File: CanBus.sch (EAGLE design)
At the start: 38 parts, among them IC1 MCP2515-I/SO, IC2 MEGA8-P, IC3 MCP2515-I/SO, Q1 16MHz, Q2 16MHz, Q3 16MHz, U1 MCP2562-E/SN, U2 MCP2562-E/SN, X1 MAC64L

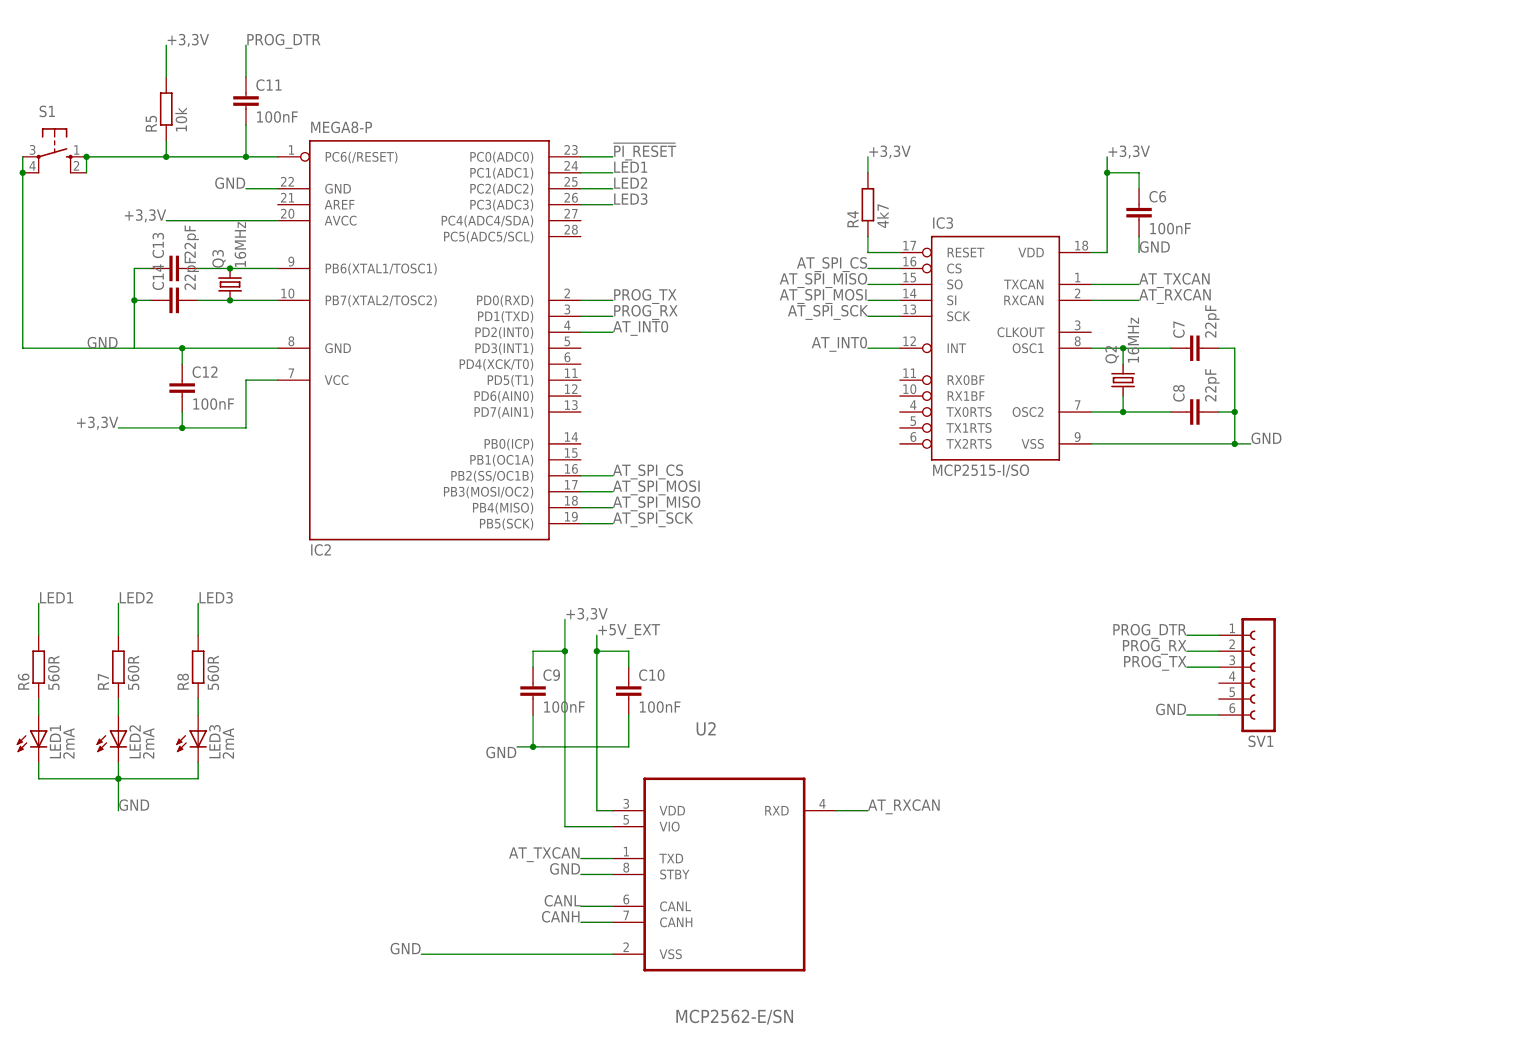
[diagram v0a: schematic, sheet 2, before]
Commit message: Platinen angepasst, Backplane
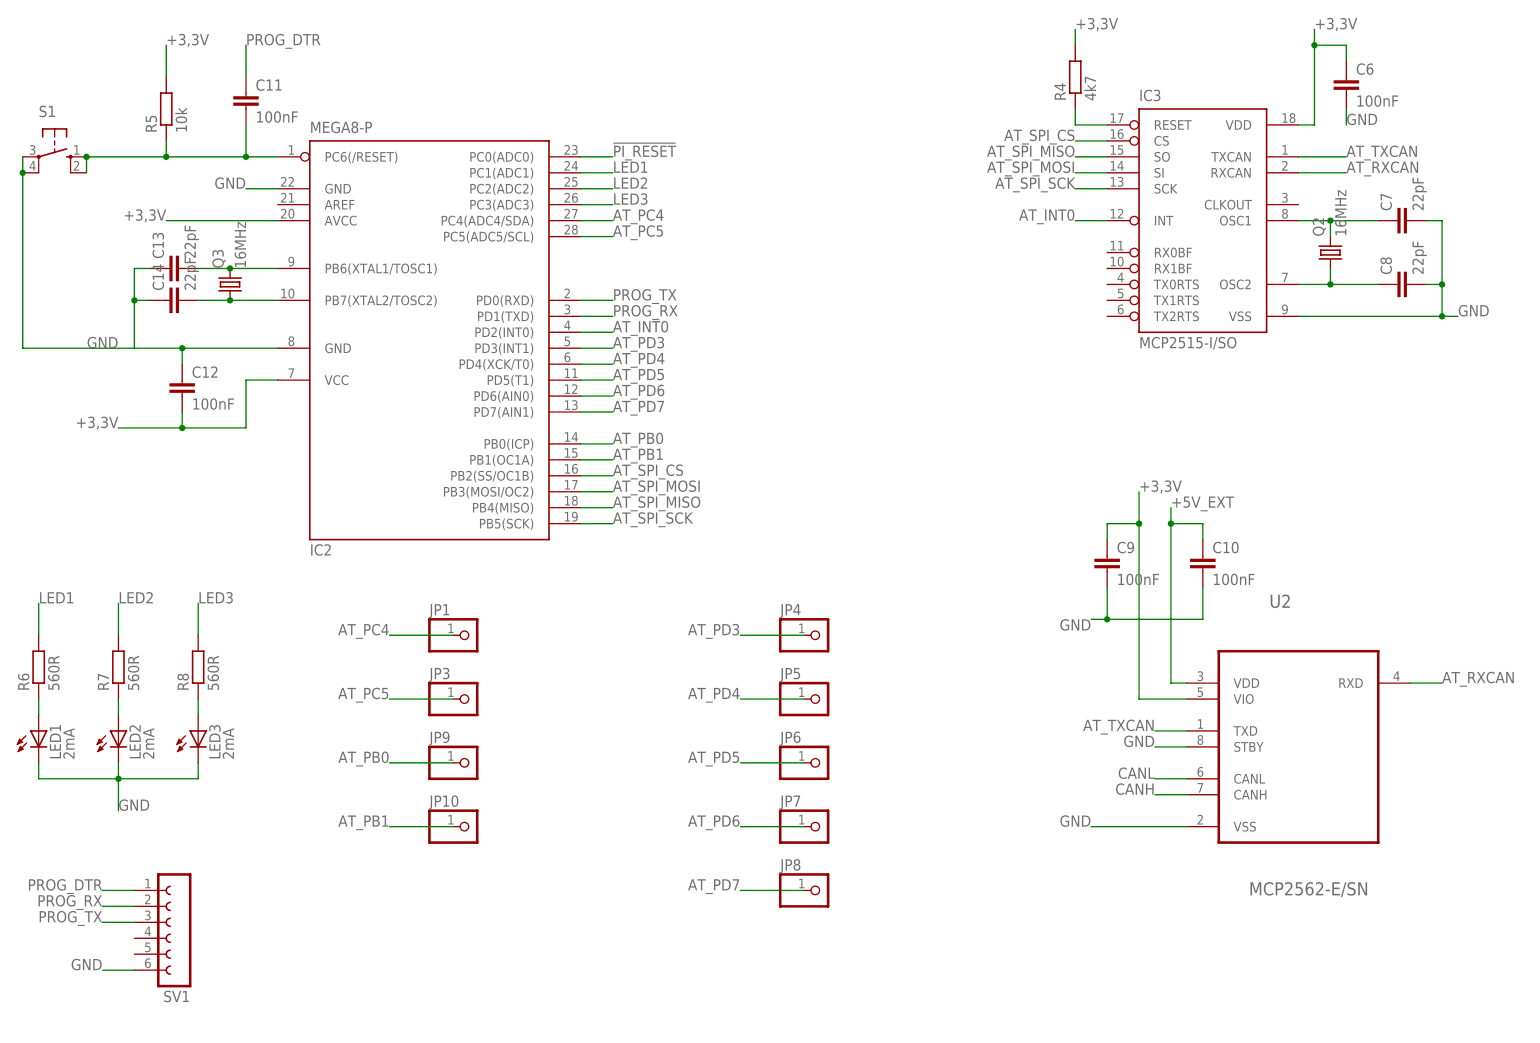
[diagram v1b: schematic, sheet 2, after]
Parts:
- added JP1, JP10, JP3, JP4, JP5, JP6, JP7, JP8, JP9: (no value), pinhead:PINHD-1X1
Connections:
- new net AT_PB0: IC2.PB0(ICP), JP9.1
- new net AT_PB1: IC2.PB1(OC1A), JP10.1
- new net AT_PC4: IC2.PC4(ADC4/SDA), JP1.1
- new net AT_PC5: IC2.PC5(ADC5/SCL), JP3.1
- new net AT_PD3: IC2.PD3(INT1), JP4.1
- new net AT_PD4: IC2.PD4(XCK/T0), JP5.1
- new net AT_PD5: IC2.PD5(T1), JP6.1
- new net AT_PD6: IC2.PD6(AIN0), JP7.1
- new net AT_PD7: IC2.PD7(AIN1), JP8.1
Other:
- moved on the sheet: C10, C6, C7, C8, C9, IC3, Q2, R4, SV1, U2
